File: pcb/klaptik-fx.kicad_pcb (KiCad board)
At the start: 4 copper layers, 41.6 x 24 mm, 31 parts, among them J1 QWIIC, J2 TagConnect, J4 Conn_01x06, J5 IO_B, J6 IO_A, U1 STM32G0xxFx, U2 LCD12864, U3 M95M01-DF

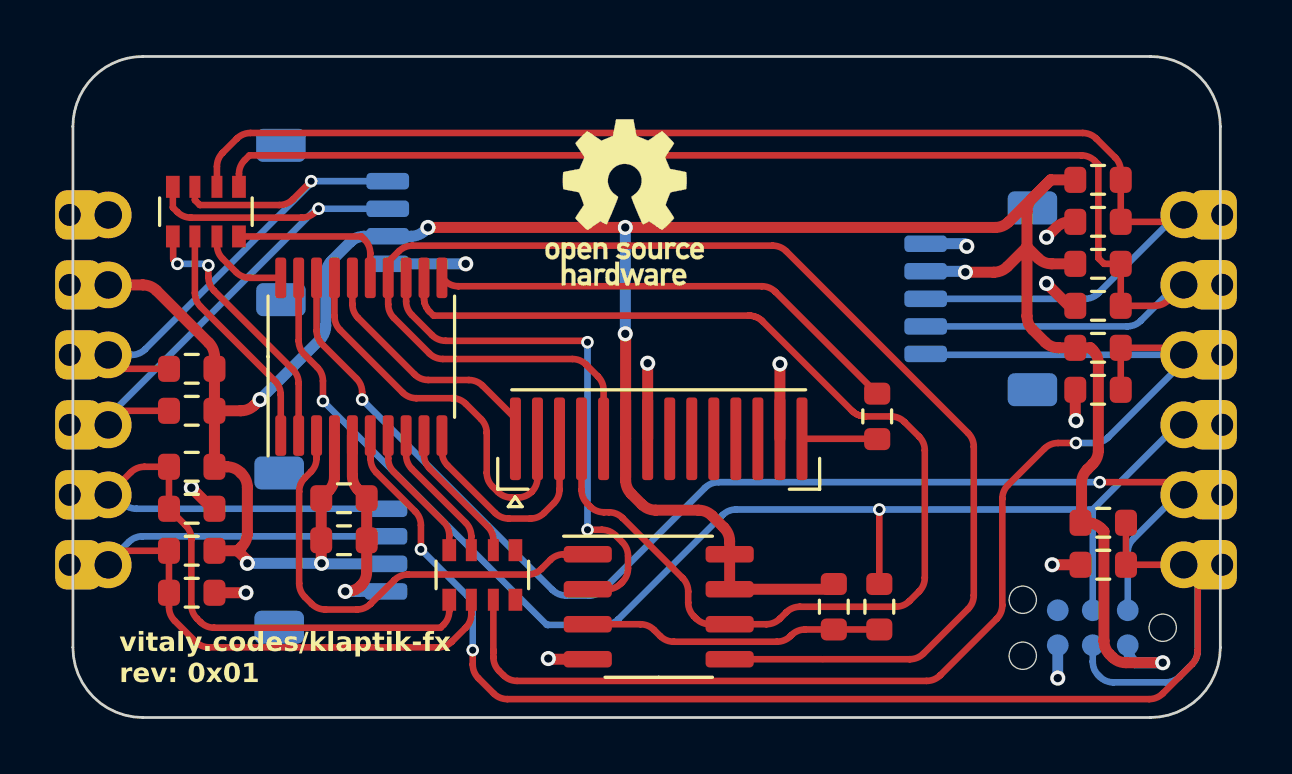
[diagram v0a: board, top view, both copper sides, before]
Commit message: pcb rev 0x02
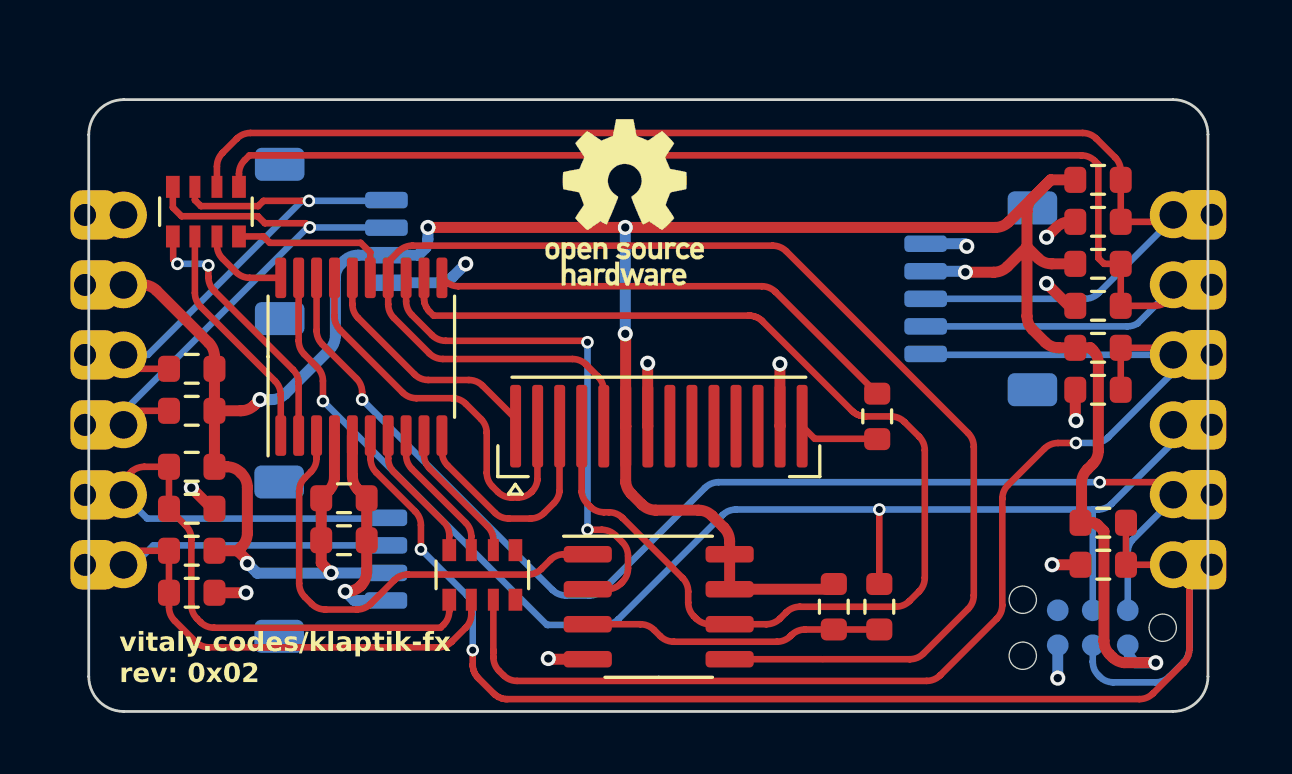
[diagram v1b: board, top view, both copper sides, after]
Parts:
- moved J1 0.69 mm to (118.7, 97.0)
- moved J4 0.55 mm to (111.1, 102.4)
- moved U2 0.46 mm to (130.6, 104.2)
- moved locked 0.38 mm to (149.2, 102.4)
- moved J6 0.33 mm to (118.7, 108.5)
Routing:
- net VDD: track 109.6 -> 110.2 mm
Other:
- board size 41.6 x 24 mm -> 40.6 x 22.2 mm
- board text added: "GPIO A"
- board text added: "GPIO B"
- board text added: "vitaly.codes/klaptik-fx rev: 0x02"
- board text removed: "GPIO_A"
- board text removed: "GPIO_B"
- board text removed: "vitaly.codes/klaptik-fx rev: 0x01"
